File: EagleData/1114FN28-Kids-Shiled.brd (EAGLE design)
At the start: 86 x 53 mm, 19 parts

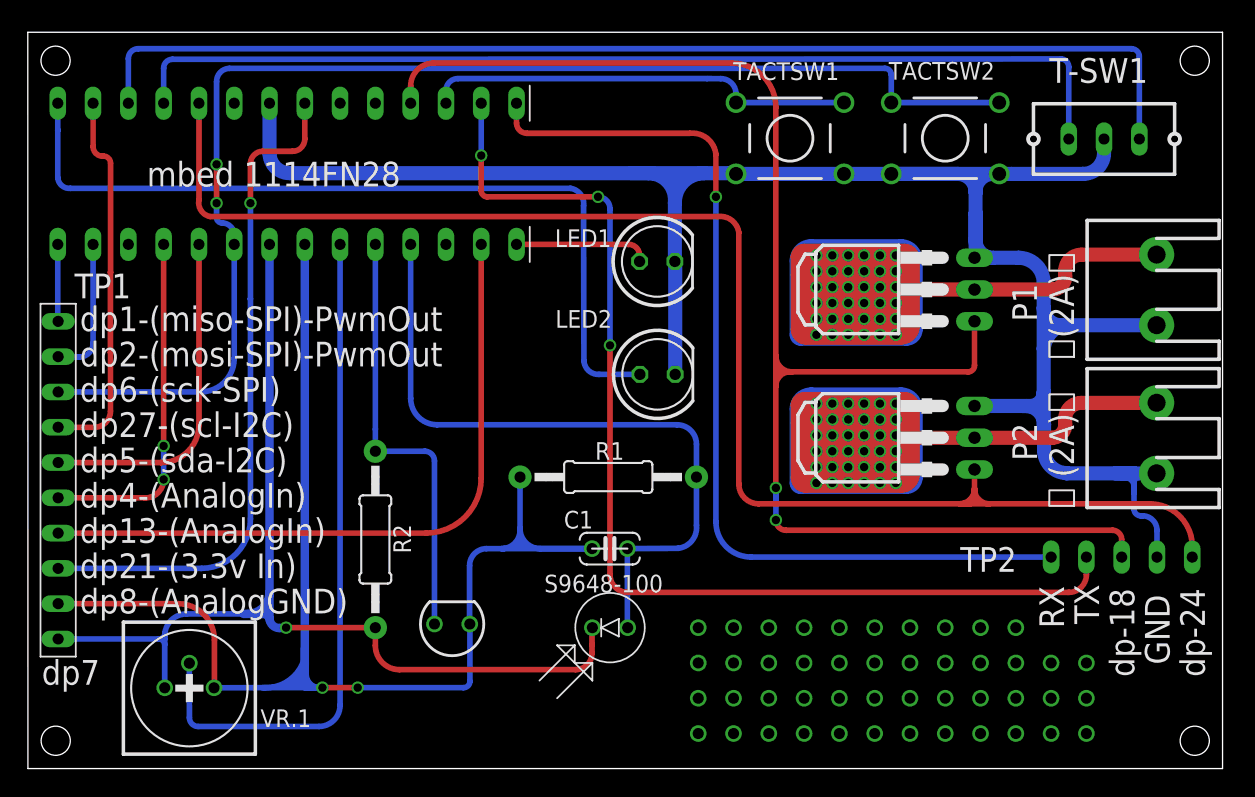
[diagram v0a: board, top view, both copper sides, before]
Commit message: Rev5
Rev5 update
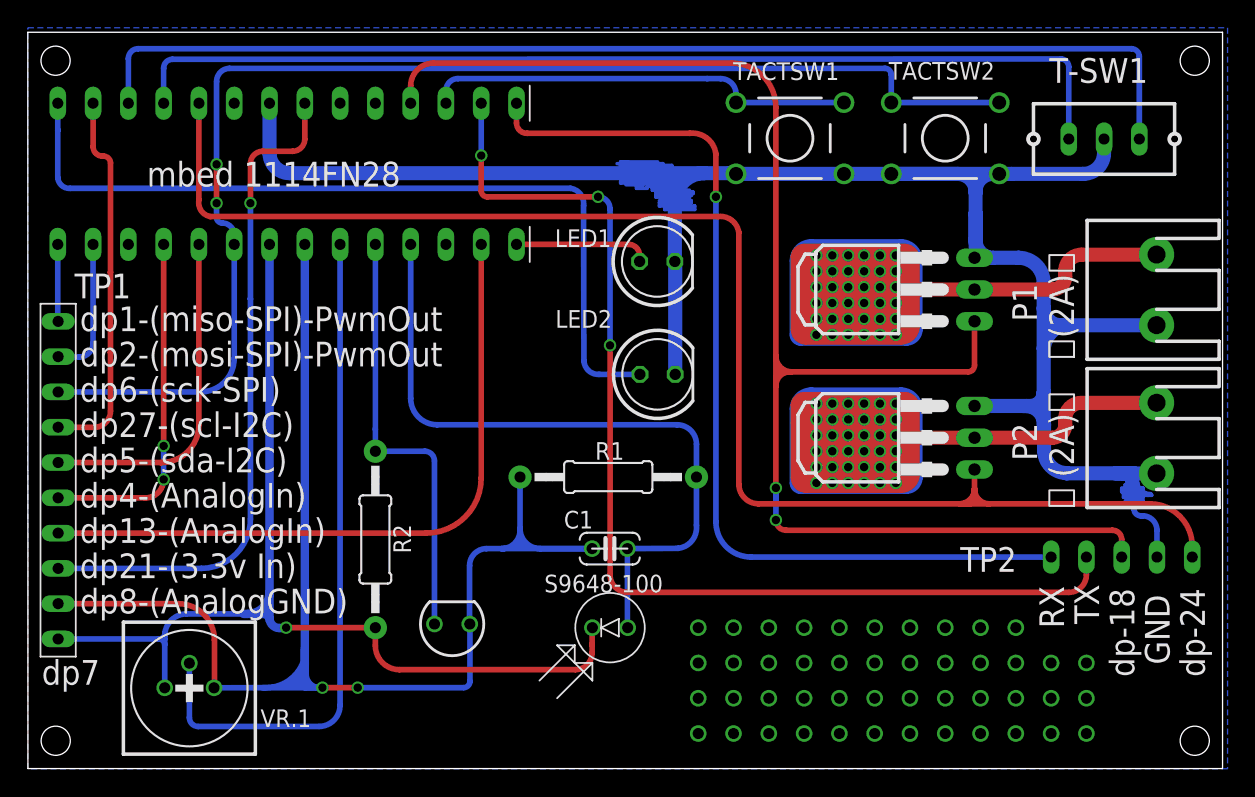
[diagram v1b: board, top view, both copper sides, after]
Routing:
- net N$4: track 0.00 -> 20.1 mm
- net N$16: track 0.00 -> 18.4 mm
- net N$23: track 0.00 -> 15.6 mm
- net N$20: track 0.00 -> 13.0 mm
- net N$24: track 0.00 -> 1.51 mm
- added copper zone on layer 16, net GND
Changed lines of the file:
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@@
 <?xml version="1.0" encoding="utf-8"?>
 <!DOCTYPE eagle SYSTEM "eagle.dtd">
-<eagle version="6.6.0">
+<eagle version="7.2.0">
 <drawing>
 <settings>
@@
 <setting verticaltext="up"/>
 </settings>
-<grid distance="50" unitdist="mil" unit="mil" style="lines" multiple="1" display="yes" altdistance="5" altunitdist="mil" altunit="mil"/>
+<grid distance="5" unitdist="mil" unit="mil" style="lines" multiple="1" display="yes" altdistance="5" altunitdist="mil" altunit="mil"/>
 <layers>
 <layer number="1" name="Top" color="4" fill="1" visible="yes" active="yes"/>
@@
 <pass name="Default">
 <param name="RoutingGrid" value="50mil"/>
+<param name="AutoGrid" value="1"/>
+<param name="Efforts" value="0"/>
+<param name="TopRouterVariant" value="1"/>
 <param name="tpViaShape" value="round"/>
 <param name="PrefDir.1" value="0"/>
@@
 <via x="76.2" y="5.08" extent="1-16" drill="0.8"/>
 <via x="76.2" y="7.62" extent="1-16" drill="0.8"/>
+<wire x1="73.66" y1="7.62" x2="76.2" y2="7.62" width="0" layer="19" extent="1-1"/>
+<wire x1="76.2" y1="5.08" x2="76.2" y2="7.62" width="0" layer="19" extent="1-1"/>
+<wire x1="71.12" y1="7.62" x2="73.66" y2="7.62" width="0" layer="19" extent="1-1"/>
+<wire x1="73.66" y1="5.08" x2="73.66" y2="7.62" width="0" layer="19" extent="1-1"/>
+<wire x1="76.2" y1="2.54" x2="76.2" y2="5.08" width="0" layer="19" extent="1-1"/>
+<wire x1="73.66" y1="2.54" x2="73.66" y2="5.08" width="0" layer="19" extent="1-1"/>
 </signal>
 <signal name="N$19">
@@
 <wire x1="80.1116" y1="18.2118" x2="80.2386" y2="18.2118" width="0.4064" layer="16"/>
 <wire x1="80.2386" y1="18.2118" x2="81.28" y2="17.1704" width="0.4064" layer="16" curve="-90"/>
+<polygon width="0.4064" layer="16" isolate="0.4064">
+<vertex x="0" y="53.34"/>
+<vertex x="86.36" y="53.34"/>
+<vertex x="86.36" y="0"/>
+<vertex x="0" y="0"/>
+</polygon>
 </signal>
 <signal name="N$6">
@@
 <wire x1="19.939" y1="45.339" x2="19.939" y2="47.9098" width="0.4064" layer="1"/>
 </signal>
+<signal name="N$4">
+<wire x1="42.418" y1="43.561" x2="45.72" y2="43.561" width="0.254" layer="16"/>
+<wire x1="45.72" y1="43.561" x2="45.72" y2="43.434" width="0.254" layer="16"/>
+<wire x1="45.72" y1="43.434" x2="42.799" y2="43.434" width="0.254" layer="16"/>
+<wire x1="45.72" y1="43.434" x2="46.355" y2="43.434" width="0.254" layer="16"/>
+<wire x1="46.355" y1="43.434" x2="46.355" y2="43.307" width="0.254" layer="16"/>
+<wire x1="46.355" y1="43.307" x2="43.18" y2="43.307" width="0.254" layer="16"/>
+<wire x1="43.18" y1="43.307" x2="43.18" y2="43.688" width="0.254" layer="16"/>
+<wire x1="43.18" y1="43.688" x2="45.339" y2="43.688" width="0.254" layer="16"/>
+<wire x1="43.18" y1="43.688" x2="42.926" y2="43.688" width="0.254" layer="16"/>
+<wire x1="42.672" y1="43.688" x2="42.672" y2="43.434" width="0.254" layer="16"/>
+<wire x1="42.672" y1="43.434" x2="42.926" y2="43.434" width="0.254" layer="16"/>
+<wire x1="42.926" y1="43.434" x2="42.926" y2="43.688" width="0.254" layer="16"/>
+<wire x1="42.926" y1="43.688" x2="42.672" y2="43.688" width="0.254" layer="16"/>
+<wire x1="42.672" y1="43.434" x2="42.672" y2="42.418" width="0.254" layer="16"/>
+<wire x1="42.672" y1="42.418" x2="43.815" y2="42.418" width="0.254" layer="16"/>
+<wire x1="43.815" y1="42.418" x2="43.815" y2="41.783" width="0.254" layer="16"/>
+<wire x1="43.815" y1="41.783" x2="44.577" y2="41.783" width="0.254" layer="16"/>
+<wire x1="44.577" y1="41.783" x2="44.577" y2="42.164" width="0.254" layer="16"/>
+<wire x1="44.577" y1="42.164" x2="42.672" y2="42.164" width="0.254" layer="16"/>
+<wire x1="42.672" y1="42.164" x2="42.672" y2="42.291" width="0.254" layer="16"/>
+</signal>
+<signal name="N$16">
+<wire x1="43.942" y1="42.037" x2="43.053" y2="42.037" width="0.254" layer="16"/>
+<wire x1="44.323" y1="42.037" x2="43.942" y2="42.037" width="0.254" layer="16"/>
+<wire x1="43.942" y1="42.037" x2="43.942" y2="42.291" width="0.254" layer="16"/>
+<wire x1="43.942" y1="42.291" x2="44.704" y2="42.291" width="0.254" layer="16"/>
+<wire x1="44.831" y1="42.291" x2="44.704" y2="42.291" width="0.254" layer="16"/>
+<wire x1="44.704" y1="42.291" x2="44.704" y2="42.037" width="0.254" layer="16"/>
+<wire x1="44.704" y1="42.037" x2="44.831" y2="42.037" width="0.254" layer="16"/>
+<wire x1="45.466" y1="42.037" x2="44.831" y2="42.037" width="0.254" layer="16"/>
+<wire x1="44.831" y1="42.037" x2="44.831" y2="41.91" width="0.254" layer="16"/>
+<wire x1="45.974" y1="41.91" x2="44.831" y2="41.91" width="0.254" layer="16"/>
+<wire x1="44.831" y1="42.037" x2="44.831" y2="42.291" width="0.254" layer="16"/>
+<wire x1="44.831" y1="42.291" x2="45.72" y2="42.291" width="0.254" layer="16"/>
+<wire x1="45.72" y1="42.291" x2="45.72" y2="42.164" width="0.254" layer="16"/>
+<wire x1="45.72" y1="42.164" x2="44.958" y2="42.164" width="0.254" layer="16"/>
+<wire x1="44.958" y1="42.164" x2="44.958" y2="41.656" width="0.254" layer="16"/>
+<wire x1="44.958" y1="41.656" x2="45.212" y2="41.656" width="0.254" layer="16"/>
+<wire x1="47.625" y1="41.656" x2="45.212" y2="41.656" width="0.254" layer="16"/>
+<wire x1="45.212" y1="41.656" x2="45.212" y2="41.529" width="0.254" layer="16"/>
+<wire x1="45.212" y1="41.529" x2="47.879" y2="41.529" width="0.254" layer="16"/>
+<wire x1="47.879" y1="41.529" x2="47.879" y2="41.402" width="0.254" layer="16"/>
+<wire x1="47.879" y1="41.402" x2="47.752" y2="41.402" width="0.254" layer="16"/>
+<wire x1="47.752" y1="41.402" x2="47.752" y2="41.275" width="0.254" layer="16"/>
+<wire x1="47.752" y1="41.275" x2="45.212" y2="41.275" width="0.254" layer="16"/>
+<wire x1="45.212" y1="41.275" x2="45.212" y2="41.402" width="0.254" layer="16"/>
+<wire x1="45.212" y1="41.275" x2="45.212" y2="41.148" width="0.254" layer="16"/>
+<wire x1="45.212" y1="41.148" x2="47.625" y2="41.148" width="0.254" layer="16"/>
+<wire x1="47.625" y1="41.148" x2="47.625" y2="41.021" width="0.254" layer="16"/>
+</signal>
+<signal name="N$20">
+<wire x1="45.466" y1="40.894" x2="47.752" y2="40.894" width="0.254" layer="16"/>
+<wire x1="47.752" y1="40.894" x2="47.752" y2="40.767" width="0.254" layer="16"/>
+<wire x1="47.752" y1="40.767" x2="45.466" y2="40.767" width="0.254" layer="16"/>
+<wire x1="45.466" y1="40.767" x2="45.466" y2="40.513" width="0.254" layer="16"/>
+<wire x1="45.466" y1="40.513" x2="48.006" y2="40.513" width="0.254" layer="16"/>
+<wire x1="48.006" y1="40.513" x2="48.006" y2="40.259" width="0.254" layer="16"/>
+<wire x1="48.006" y1="40.259" x2="45.847" y2="40.259" width="0.254" layer="16"/>
+<wire x1="45.847" y1="40.259" x2="45.847" y2="40.386" width="0.254" layer="16"/>
+<wire x1="45.847" y1="40.386" x2="46.99" y2="40.386" width="0.254" layer="16"/>
+<wire x1="46.99" y1="40.386" x2="46.99" y2="42.164" width="0.254" layer="16"/>
+</signal>
+<signal name="N$23">
+<wire x1="78.994" y1="19.304" x2="80.264" y2="19.304" width="0.254" layer="16"/>
+<wire x1="80.264" y1="19.304" x2="80.264" y2="19.558" width="0.254" layer="16"/>
+<wire x1="80.264" y1="19.558" x2="78.867" y2="19.558" width="0.254" layer="16"/>
+<wire x1="78.867" y1="19.558" x2="78.867" y2="19.812" width="0.254" layer="16"/>
+<wire x1="80.137" y1="19.812" x2="78.867" y2="19.812" width="0.254" layer="16"/>
+<wire x1="78.867" y1="19.812" x2="78.867" y2="19.939" width="0.254" layer="16"/>
+<wire x1="78.867" y1="19.939" x2="80.137" y2="19.939" width="0.254" layer="16"/>
+<wire x1="78.867" y1="19.939" x2="78.74" y2="19.939" width="0.254" layer="16"/>
+<wire x1="78.74" y1="19.939" x2="78.74" y2="20.193" width="0.254" layer="16"/>
+<wire x1="78.74" y1="20.193" x2="80.264" y2="20.193" width="0.254" layer="16"/>
+<wire x1="80.264" y1="20.193" x2="80.264" y2="20.066" width="0.254" layer="16"/>
+<wire x1="80.264" y1="20.066" x2="78.994" y2="20.066" width="0.254" layer="16"/>
+<wire x1="78.994" y1="20.066" x2="78.994" y2="20.447" width="0.254" layer="16"/>
+<wire x1="78.994" y1="20.447" x2="79.883" y2="20.447" width="0.254" layer="16"/>
+<wire x1="79.883" y1="20.447" x2="79.883" y2="20.32" width="0.254" layer="16"/>
+<wire x1="79.883" y1="20.701" x2="79.883" y2="20.574" width="0.254" layer="16"/>
+<wire x1="79.883" y1="20.574" x2="80.264" y2="20.193" width="0.254" layer="16" curve="90"/>
+<wire x1="79.883" y1="20.574" x2="80.645" y2="19.812" width="0.254" layer="16" curve="90"/>
+<wire x1="80.264" y1="20.193" x2="80.645" y2="19.812" width="0.254" layer="16" curve="90"/>
+<wire x1="80.645" y1="19.812" x2="80.772" y2="19.812" width="0.254" layer="16"/>
+<wire x1="80.772" y1="19.812" x2="80.899" y2="19.685" width="0.254" layer="16" curve="-90"/>
+<wire x1="80.899" y1="19.685" x2="80.137" y2="19.685" width="0.254" layer="16"/>
+<wire x1="80.137" y1="19.685" x2="79.121" y2="20.701" width="0.254" layer="16" curve="-90"/>
+<wire x1="79.121" y1="20.701" x2="79.375" y2="20.701" width="0.254" layer="16"/>
+</signal>
+<signal name="N$24">
+<wire x1="79.756" y1="20.828" x2="79.756" y2="20.574" width="0.254" layer="16"/>
+<wire x1="79.756" y1="20.574" x2="80.645" y2="19.685" width="0.254" layer="16" curve="90"/>
+</signal>
 </signals>
